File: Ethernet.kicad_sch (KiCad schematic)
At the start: 20 parts, among them T1 WE-RJ45_7499010211A, U4 DP83825IRMQR, Y2 ECS-250-12-33-AGN-TR

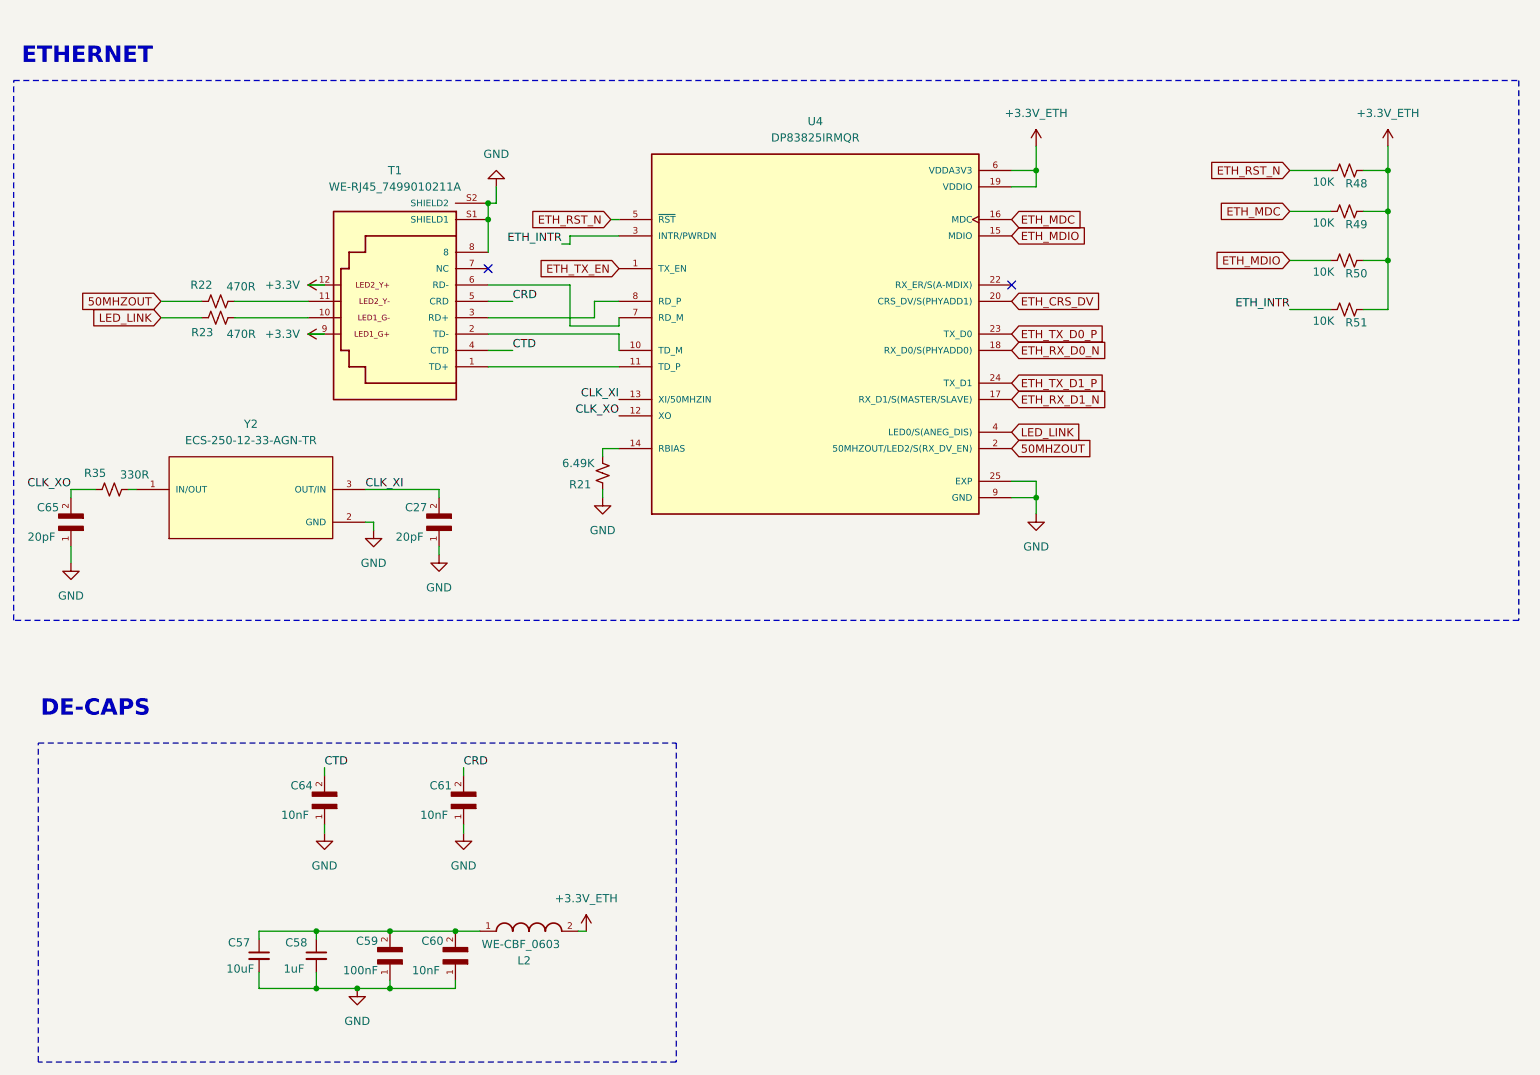
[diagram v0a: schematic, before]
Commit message: new
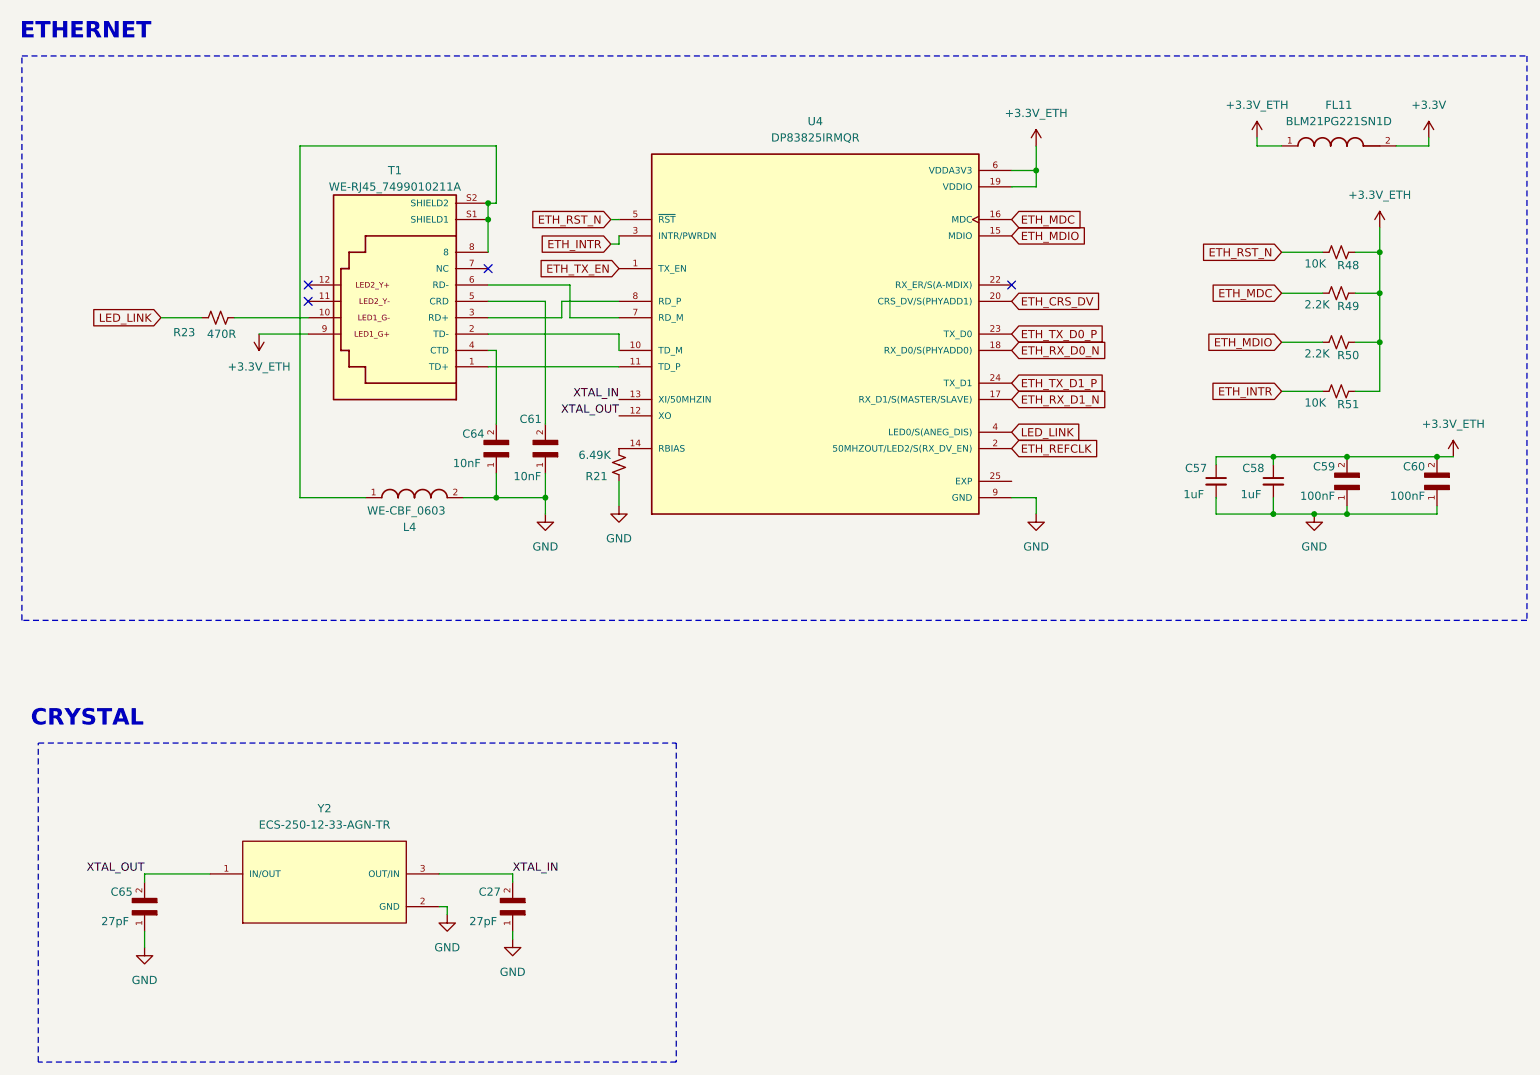
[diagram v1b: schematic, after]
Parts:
- removed L2: WE-CBF_0603, GNSS_Library:WE-CBF_0603_W2.6, symbol WE-CBF_0603:WE-CBF_0603
- removed R22: 470R, symbol Device:R_Small_US
- removed R35: 330R, symbol Device:R_Small_US
- added FL11: BLM21PG221SN1D, BLM21PG221SN1D:BEADC2012X105N, symbol BLM21PG221SN1D:BLM21PG221SN1D
- added L4: WE-CBF_0603, GNSS_Library:WE-CBF_0603_W2.6, symbol WE-CBF_0603:WE-CBF_0603
- C27, C65: value 20pF -> 27pF
- C57: value 10uF -> 1uF
- C60: value 10nF -> 100nF
- R49, R50: value 10K -> 2.2K
- T1: footprint Module:7499010211A -> GNSS:7499010211A
- U4: footprint GNSS_Library:XCVR_DP83825IRMQR -> GNSS:XCVR_DP83825IRMQR
- Y2: footprint GNSS_Library:XTAL_ECS-250-12-33-AGN-TR -> GNSS:XTAL_ECS-250-12-33-AGN-TR
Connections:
- net CLK_XO is gone; now on net XTAL_OUT: C65.2, U4.12 (XO)
- net +3.3V: now also FL11.2; no longer T1.12, T1.9
- net +3.3V_ETH: now also C57.1, C58.1, C59.2, C60.2, T1.9, FL11.1
- net EXP: no longer C27.1, C57.2, C58.2, C59.1, C60.1, C61.1, C64.1, C65.1, R21.1, T1.8, T1.S1 (SHIELD1), T1.S2 (SHIELD2), U4.21 (GND), U4.9 (GND), Y2.2 (GND), Y2.4 (GND)
- net XTAL_OUT: now reaches Y2.1 (IN/OUT)
- net 50MHZOUT renamed ETH_REFCLK
- net CLK_XI renamed XTAL_IN
- net CRD: no longer names the net of C61.2, T1.5 (CRD)
- net CTD: no longer names the net of C64.2, T1.4 (CTD)
- new net: L4.1, T1.8, T1.S1 (SHIELD1), T1.S2 (SHIELD2)
- new net GND: C27.1, C57.2, C58.2, C59.1, C60.1, C61.1, C64.1, C65.1, L4.2, R21.1, U4.21 (GND), U4.9 (GND), Y2.2 (GND), Y2.4 (GND)
- no-connect marks 2 -> 4
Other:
- note added: "CRYSTAL"
- note removed: "DE-CAPS"
- moved on the sheet: C27, C57, C58, C59, C60, C61, C64, C65, R21, R48, R49, R50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
